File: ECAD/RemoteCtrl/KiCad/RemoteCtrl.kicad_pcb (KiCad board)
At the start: 2 copper layers, 101.6 x 81.3 mm, 83 parts, among them J1 UI, SW1 MX1A-E1NW, SW2 MX1A-E1NW, SW3 MX1A-E1NW, SW4 MX1A-E1NW, SW5 MX1A-E1NW, SW6 MX1A-E1NW, SW7 MX1A-E1NW, SW8 MX1A-E1NW, U1 74LVC1G17, U2 74LVC1G17, U3 74LVC1G17, U4 74LVC1G17, U5 74LVC1G17, U6 74LVC1G17, U7 74LVC1G17, U8 74LVC1G17

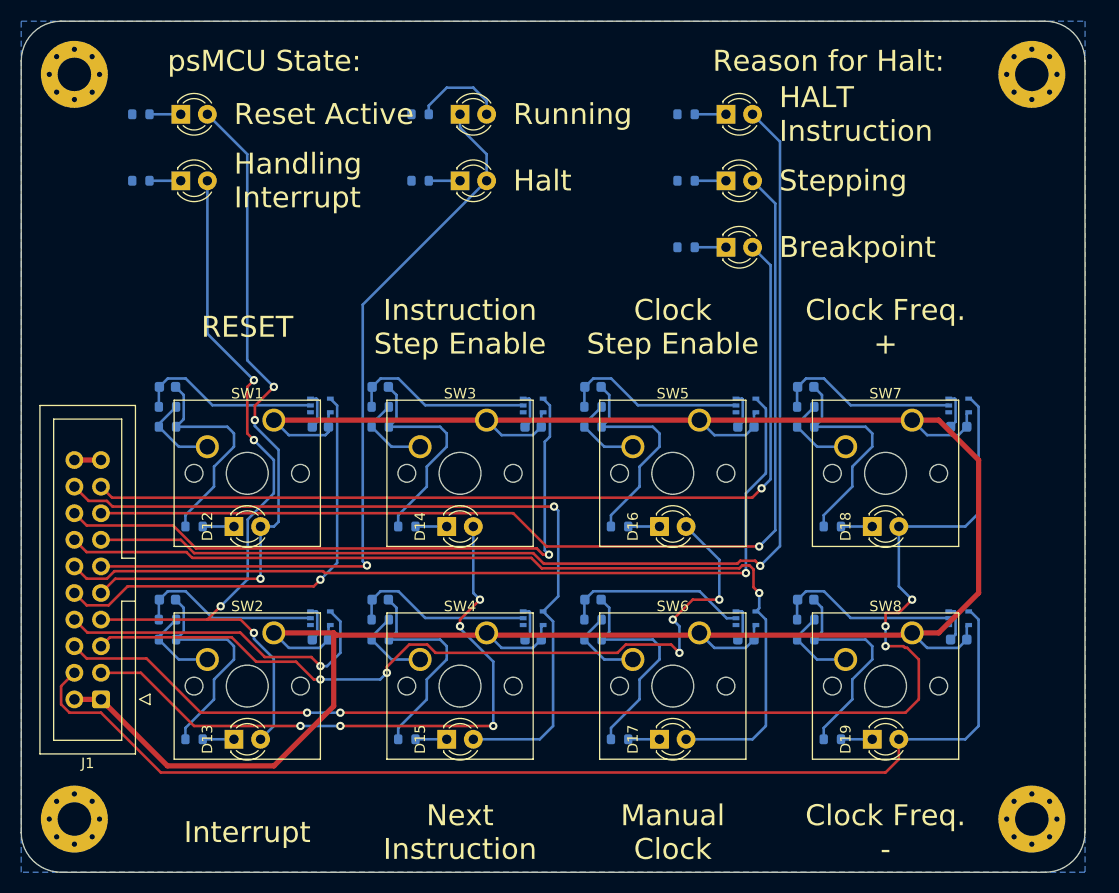
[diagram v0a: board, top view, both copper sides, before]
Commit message: Remote control work.
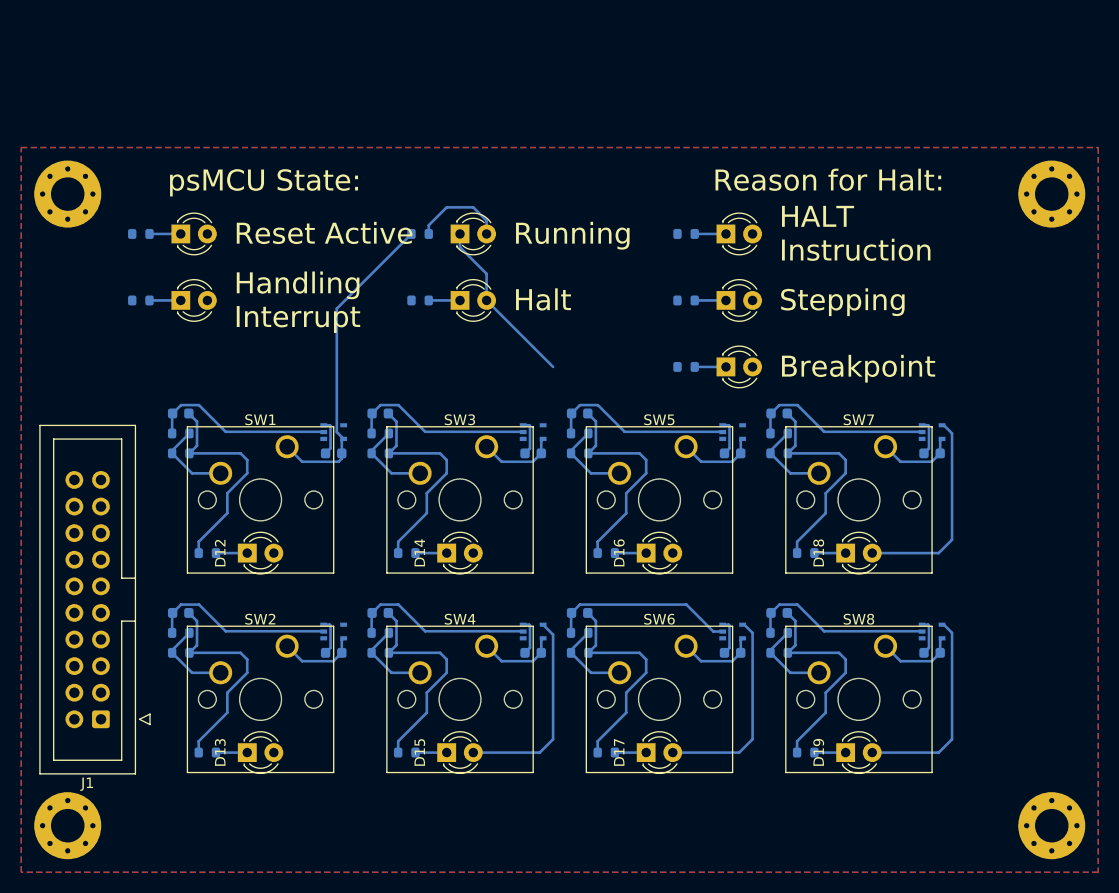
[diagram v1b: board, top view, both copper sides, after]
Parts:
- moved H2 11.6 mm to (191.1, 44.5)
- moved H1 11.4 mm to (97.2, 44.5)
- moved D1 11.4 mm to (108.0, 48.3)
- moved D10 11.4 mm to (160.0, 54.6)
- moved D11 11.4 mm to (160.0, 61.0)
- moved D2 11.4 mm to (108.0, 54.6)
- moved D7 11.4 mm to (134.6, 54.6)
- moved D8 11.4 mm to (134.6, 48.3)
- moved D9 11.4 mm to (160.0, 48.3)
- moved R1 11.4 mm to (104.1, 48.3)
- moved R10 11.4 mm to (156.2, 54.6)
- moved R11 11.4 mm to (156.2, 61.0)
- moved R2 11.4 mm to (104.1, 54.6)
- moved R7 11.4 mm to (130.8, 54.6)
- moved R8 11.4 mm to (130.8, 48.3)
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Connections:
- R8 pad 2: GND -> +5V
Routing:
- net +5V: track 248.5 -> 83.9 mm
- net /LED_Halted_Inst: track 109.2 -> 0.00 mm, vias 1 -> 0
- net /BTN_INC_CLK_F: track 124.6 -> 19.6 mm, vias 5 -> 0
- net /LED_Halted_Step: track 100.6 -> 0.00 mm, vias 1 -> 0
- net /BTN_DEC_CLK_F: track 108.3 -> 19.6 mm
- net /LED_Halted_Bkpt: track 88.0 -> 0.00 mm, vias 1 -> 0
- net /BTN_CLK_STEP_EN: track 82.8 -> 0.00 mm, vias 1 -> 0
- net /LED_CLK_STEP_EN: track 76.9 -> 0.00 mm, vias 5 -> 0
- net /LED_INT_Active: track 74.3 -> 0.00 mm, vias 4 -> 0
- net /BTN_CLK_STEP: track 90.2 -> 19.6 mm, vias 1 -> 0
- net /RESET: track 65.9 -> 0.00 mm, vias 3 -> 0
- net /BTN_INST_STEP_EN: track 62.5 -> 0.00 mm, vias 1 -> 0
- net /LED_INST_STEP_EN: track 61.0 -> 0.00 mm, vias 5 -> 0
- net /LED_Halted: track 74.6 -> 16.4 mm, vias 1 -> 0
- net /BTN_INST_STEP: track 76.9 -> 19.5 mm, vias 1 -> 0
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- added copper zone on F.Cu, net +5V
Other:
- board outline removed
- board text removed: "Clock Freq. +"
- board text removed: "Clock Freq. -"
- board text removed: "Clock Step Enable"
- board text removed: "Instruction Step Enable"
- board text removed: "Interrupt"
- board text removed: "Manual Clock"
- board text removed: "Next Instruction"
- board text removed: "RESET"
